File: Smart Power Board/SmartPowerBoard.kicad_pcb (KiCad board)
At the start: 4 copper layers, 57.8 x 35.4 mm, 116 parts, among them J1 430450200, J2 USB_C_Receptacle_USB2.0_16P, J6 430450601, J7 Screw_Terminal_01x04, Q1 FDN338P, Q4 FDN335N, SW1 SW_Push, SW2 SW_Push, SW3 SW_Push, U1 INA3221, U2 TPS561201DDCR, U4 TPS56C230RJER, U5 TPS56C230RJER, U6 RP2040, U7 W25Q32JVSS, U8 TPS561201DDCR, Y1 FL1200138

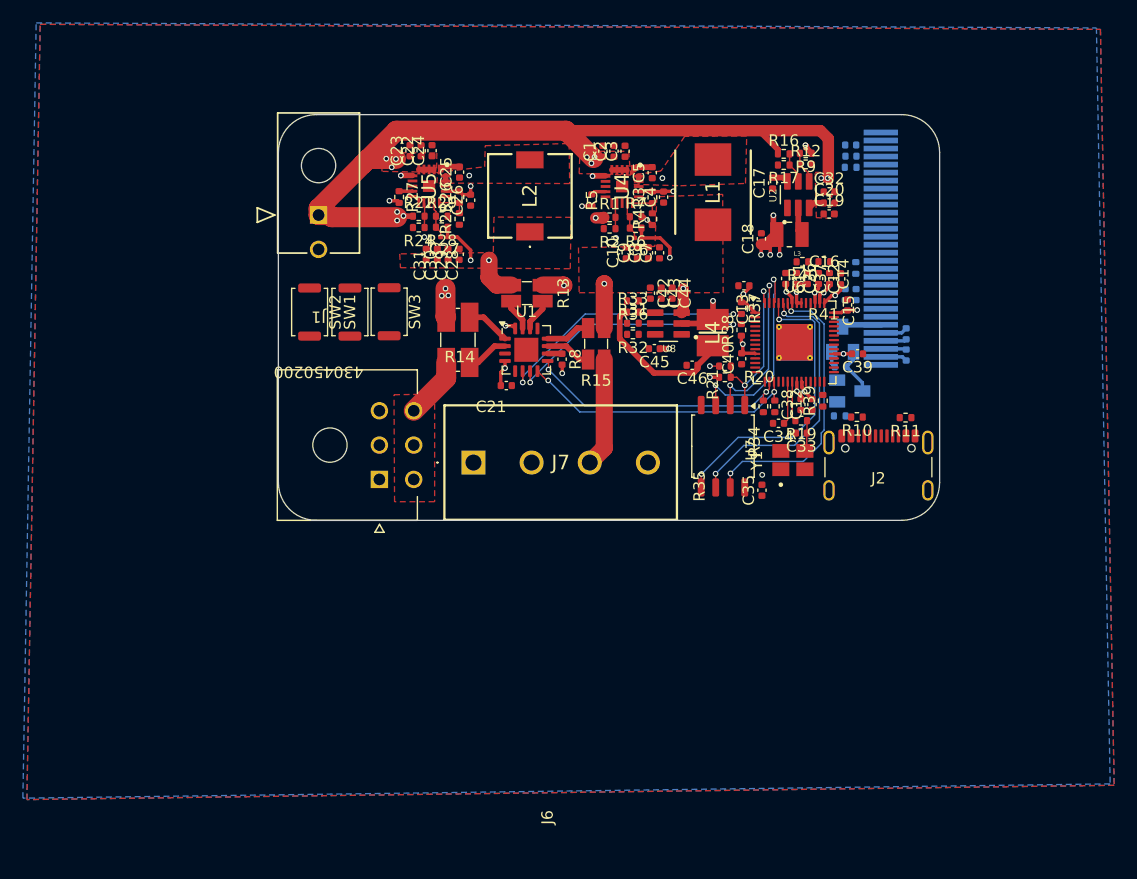
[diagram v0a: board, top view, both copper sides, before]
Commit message: Feat[SmartPowerBoard]: More Routing
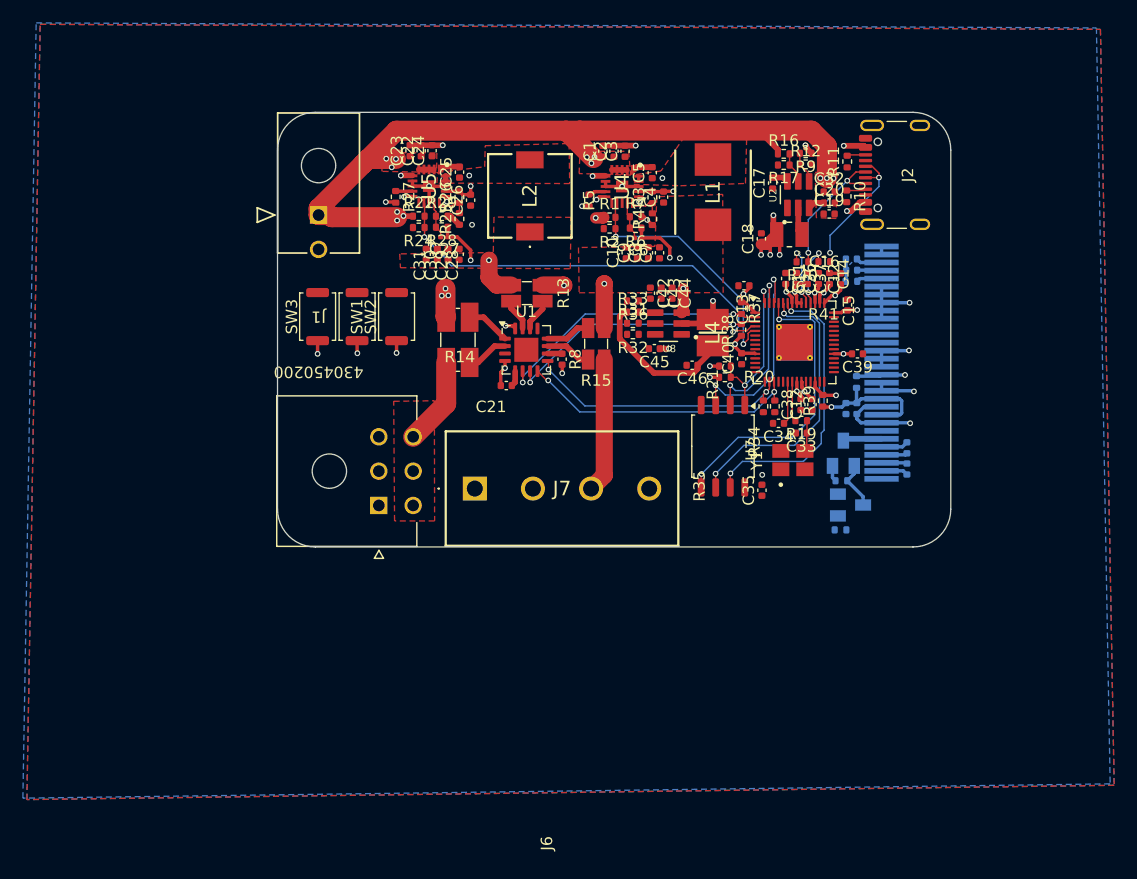
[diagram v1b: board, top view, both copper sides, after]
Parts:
- moved J2 26.6 mm to (188.6, 76.8), turned to 90 degrees
- moved R11 22.9 mm to (183.3, 75.6), turned to 90 degrees
- moved R10 19.3 mm to (183.2, 78.7), turned to -90 degrees
- moved Q4 9.96 mm to (183.6, 105.6)
- moved R18 9.96 mm to (184.1, 94.9)
- moved R43 9.96 mm to (183.7, 86.1)
- moved R44 9.96 mm to (182.7, 107.8)
- moved U9 9.96 mm to (187.1, 93.2)
- moved C47 9.96 mm to (183.2, 97.2)
- moved C48 9.96 mm to (184.1, 97.2)
- moved C49 9.96 mm to (183.7, 85.1)
- moved C50 9.96 mm to (183.7, 84.1)
- moved C51 9.96 mm to (188.5, 102.5)
- moved C52 9.96 mm to (188.5, 100.6)
- moved Q1 9.96 mm to (183.0, 101.1)
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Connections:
- J2 pad A4: /MCU/5V_{IN} -> /Buck Converter 5V/5V_{OUT}
- J2 pad A9: /MCU/5V_{IN} -> /Buck Converter 5V/5V_{OUT}
- J2 pad B4: /MCU/5V_{IN} -> /Buck Converter 5V/5V_{OUT}
- J2 pad B9: /MCU/5V_{IN} -> /Buck Converter 5V/5V_{OUT}
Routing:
- net /OLED Display/RES#: track 0.00 -> 76.3 mm, vias 0 -> 2
- net /MCU/RUN: track 0.00 -> 64.9 mm, vias 0 -> 2
- net /MCU/USB_BOOT: track 0.80 -> 45.6 mm, vias 1 -> 2
- net GND: track 1.25 -> 44.5 mm, vias 1 -> 14
- net /Buck Converter 5V/5V_{OUT}: track 10.6 -> 49.8 mm, vias 3 -> 6
- net /Buck Converter 3.3V/EN: track 2.27 -> 37.5 mm
- net /MCU/3.3V_{CC}: track 110.7 -> 139.6 mm, vias 18 -> 19
- net /Buck Converter 5V/EN: track 2.29 -> 22.1 mm, vias 0 -> 2
- net /MCU/USB_P: track 0.00 -> 12.1 mm, vias 0 -> 2
- net /MCU/USB_M: track 0.00 -> 11.3 mm, vias 0 -> 2
- net Net-(U6-USB_DM): track 0.00 -> 5.59 mm, vias 0 -> 2
- net Net-(U6-USB_DP): track 0.00 -> 5.47 mm, vias 0 -> 2
- net /Connectors/12V_{OUT}: track 5.39 -> 7.69 mm
- net Net-(U9-VCC): track 0.00 -> 2.28 mm
- net /Connectors/5V_{OUT}: track 9.53 -> 11.8 mm
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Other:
- board size 57.8 x 35.4 mm -> 58.8 x 38 mm
